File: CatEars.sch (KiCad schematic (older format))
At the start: 14 parts, among them J0 Conn_01x03_Female, J1 Conn_01x03_Female

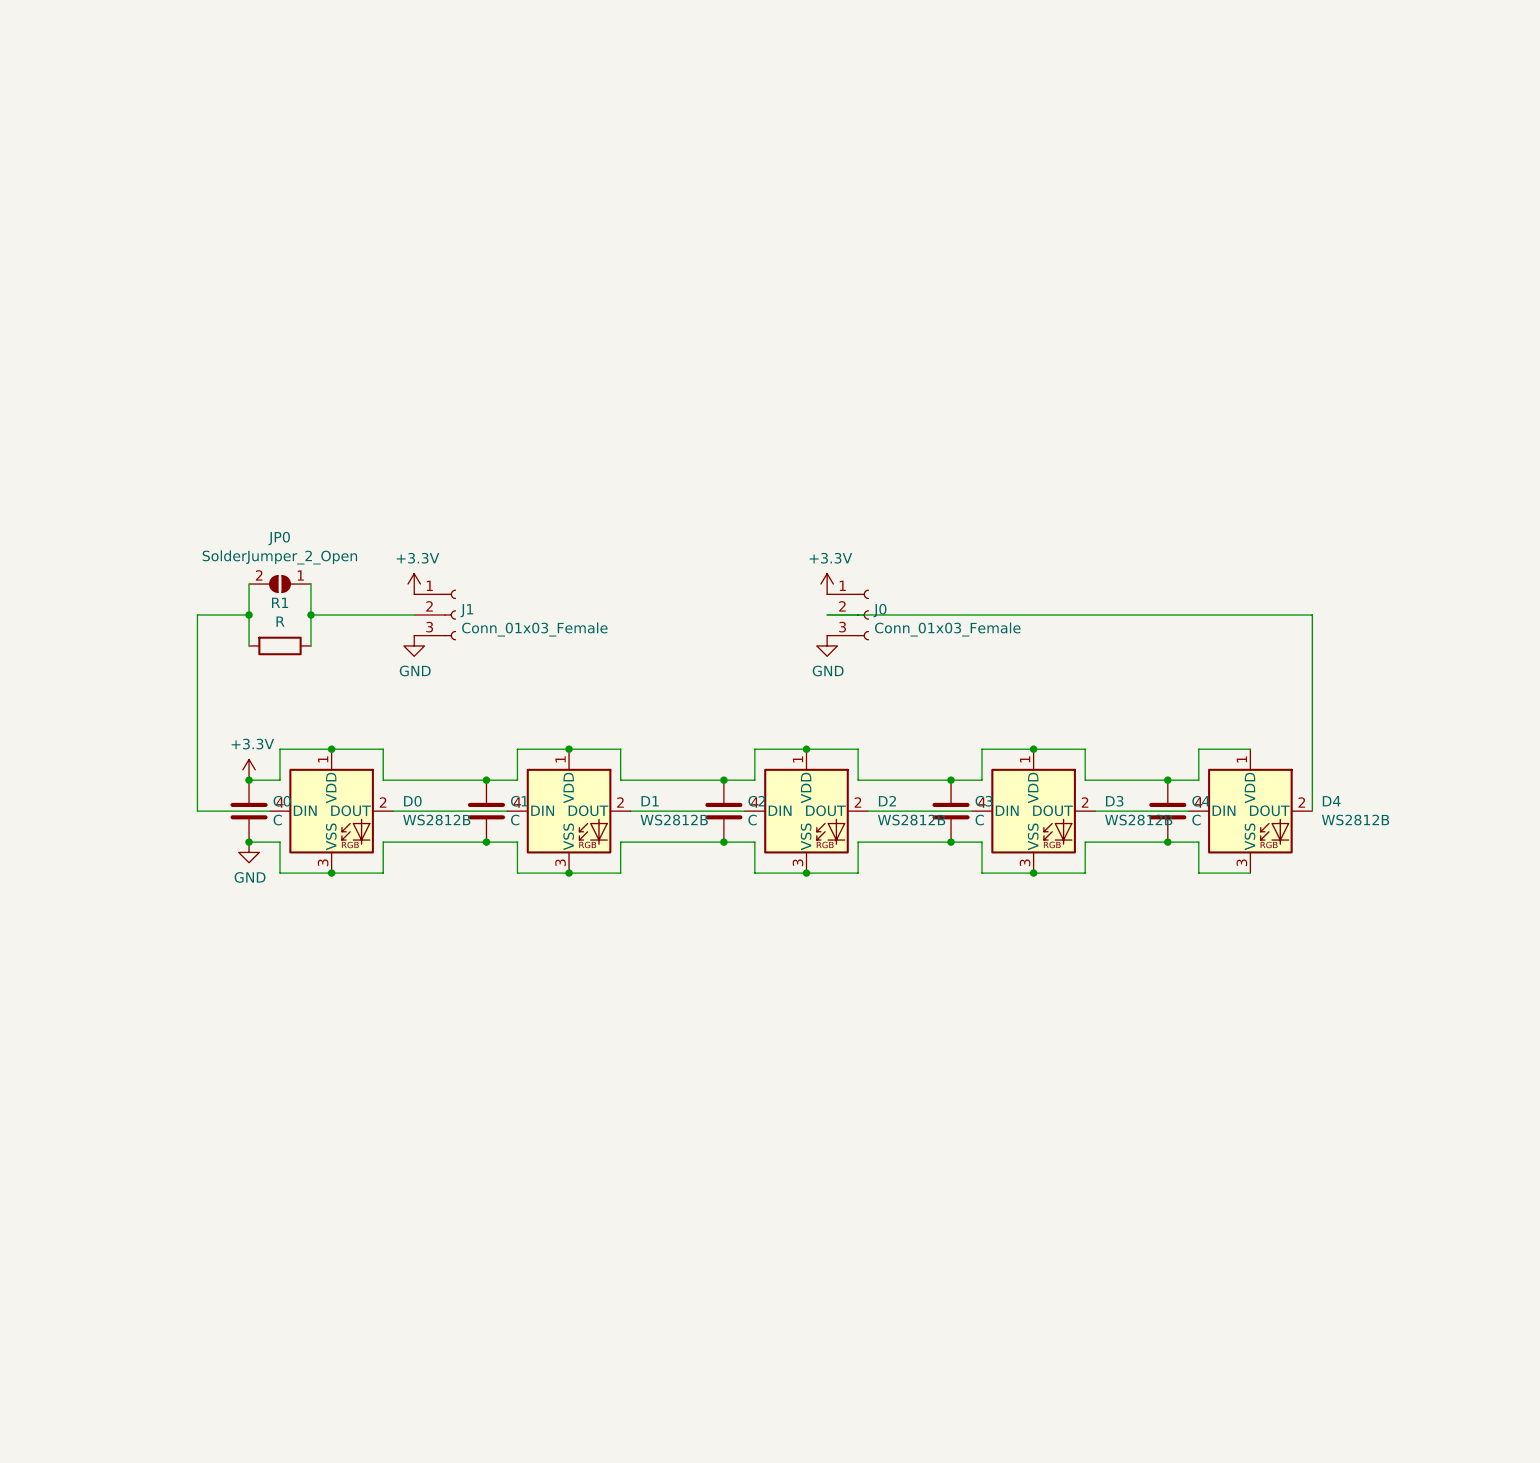
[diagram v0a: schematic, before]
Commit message: Added schematic and copper
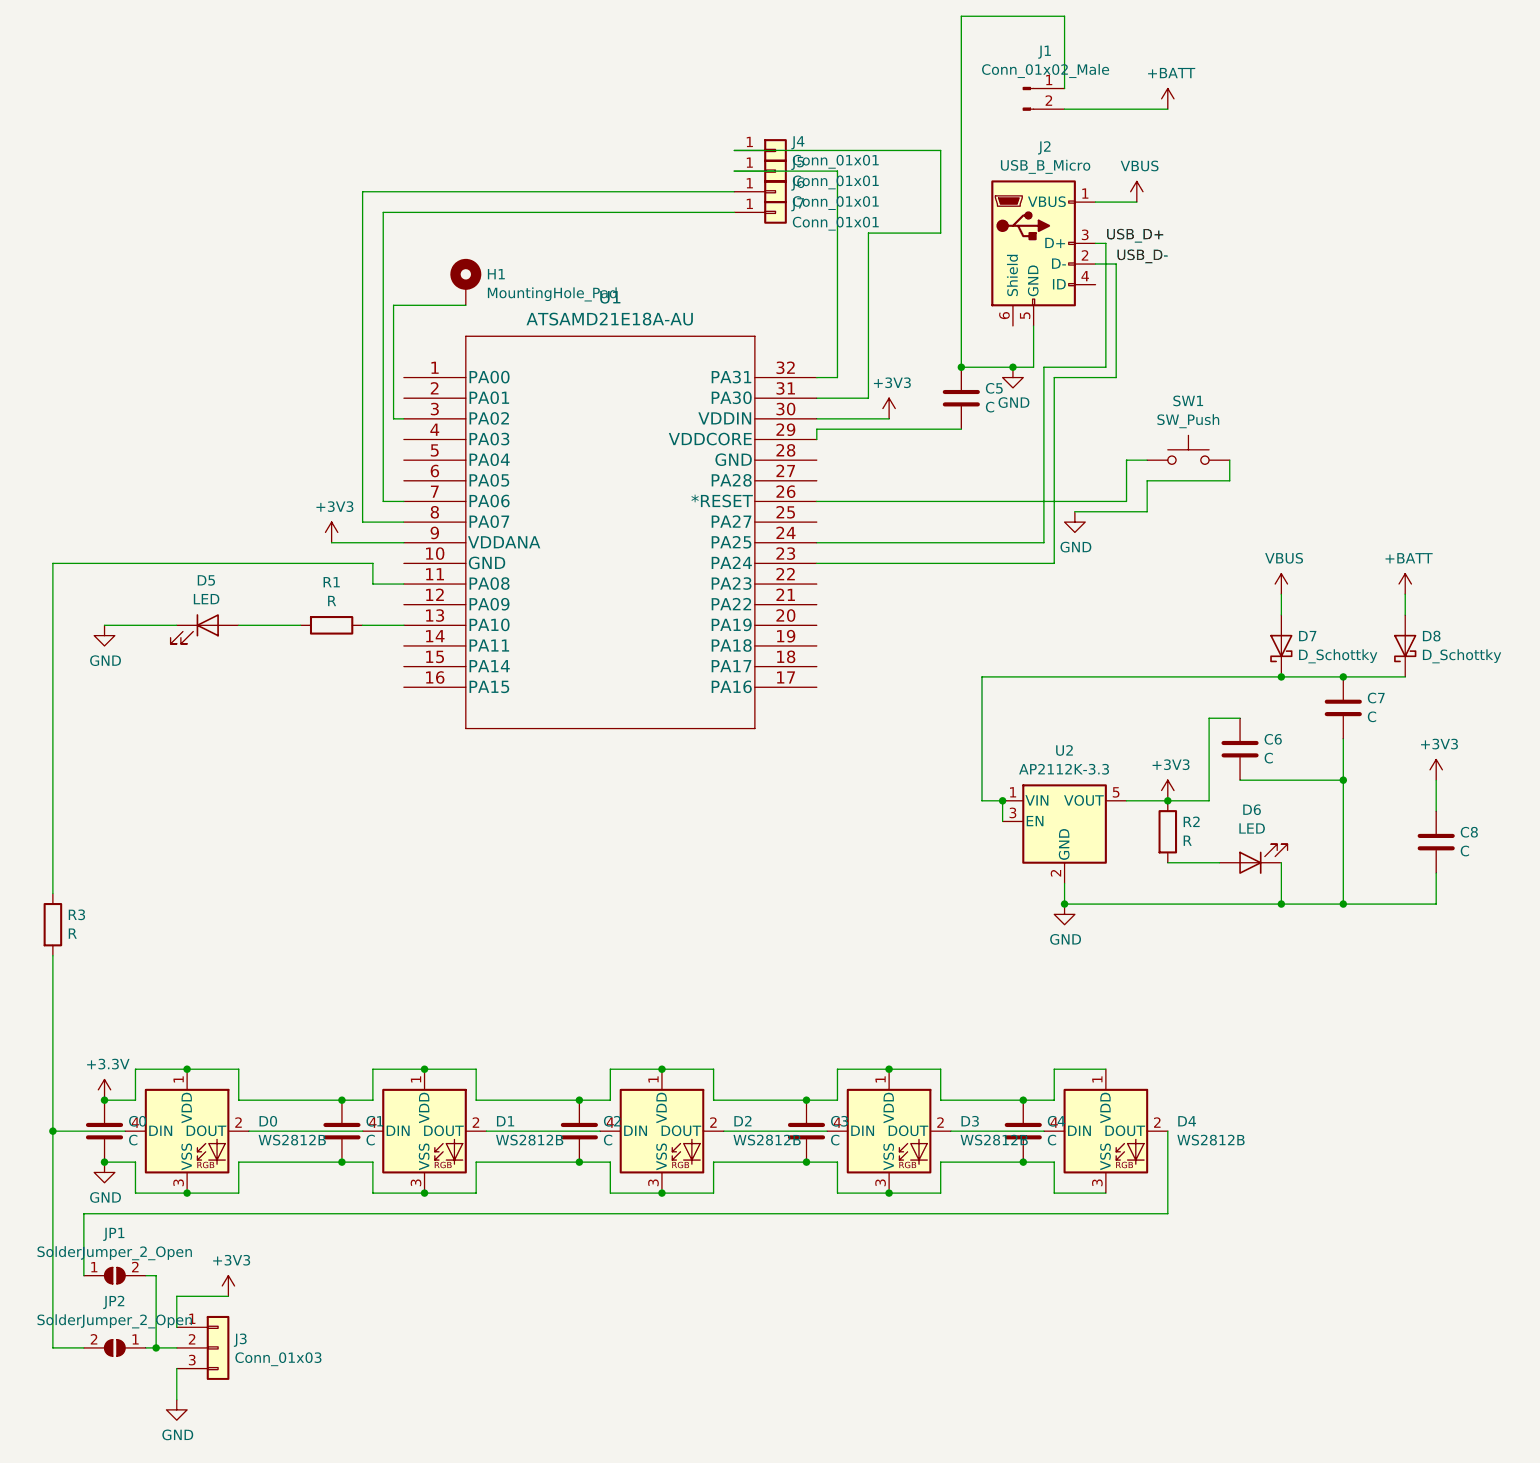
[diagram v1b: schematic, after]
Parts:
- removed J0, J1: Conn_01x03_Female, Connector_PinSocket_2.54mm:PinSocket_1x03_P2.54mm_Vertical, symbol Connector:Conn_01x03_Female
- removed JP0: SolderJumper_2_Open, Jumper:SolderJumper-2_P1.3mm_Open_TrianglePad1.0x1.5mm, symbol Jumper:SolderJumper_2_Open
- added C5, C6, C7, C8: C, Capacitor_SMD:C_0603_1608Metric_Pad1.05x0.95mm_HandSolder, symbol Device:C
- added D5, D6: LED, LED_SMD:LED_0805_2012Metric_Pad1.15x1.40mm_HandSolder, symbol Device:LED
- added D7, D8: D_Schottky, Diode_SMD:D_SOT-23_ANK, symbol Device:D_Schottky
- added H1: MountingHole_Pad, TestPoint:TestPoint_Pad_D1.5mm, symbol Mechanical:MountingHole_Pad
- added J1: Conn_01x02_Male, Connector_JST:JST_PH_B2B-PH-K_1x02_P2.00mm_Vertical, symbol Connector:Conn_01x02_Male
- added J2: USB_B_Micro, Connector_USB:USB_Micro-B_GCT_USB3076-30-A, symbol Connector:USB_B_Micro
- added J3: Conn_01x03, Connector_PinSocket_2.54mm:PinSocket_1x03_P2.54mm_Vertical, symbol Connector_Generic:Conn_01x03
- added J4, J5, J6, J7: Conn_01x01, TestPoint:TestPoint_Pad_D1.0mm, symbol Connector_Generic:Conn_01x01
- added JP1, JP2: SolderJumper_2_Open, Jumper:SolderJumper-2_P1.3mm_Open_TrianglePad1.0x1.5mm, symbol Jumper:SolderJumper_2_Open
- added R2, R3: R, Resistor_SMD:R_0805_2012Metric_Pad1.15x1.40mm_HandSolder, symbol Device:R
- added SW1: SW_Push, Button_Switch_SMD:SW_SPST_TL3342, symbol Switch:SW_Push
- added U1: ATSAMD21E18A-AU, Package_QFP:TQFP-32_7x7mm_P0.8mm, symbol 2020-01-10_20-18-23:ATSAMD21E18A-AU
- added U2: AP2112K-3.3, Package_TO_SOT_SMD:SOT-23-5, symbol Regulator_Linear:AP2112K-3.3
- R1: footprint Capacitor_SMD:C_0805_2012Metric_Pad1.15x1.40mm_HandSolder -> Resistor_SMD:R_0805_2012Metric_Pad1.15x1.40mm_HandSolder
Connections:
- net +3V3: now also C6.1, C8.1, J3.1 (Pin_1), R2.1, U1.30 (VDDIN), U1.9 (VDDANA), U2.5 (VOUT)
- net GND: now also C5.1, C6.2, C7.2, C8.2, D5.1 (K), D6.1 (K), J1.1 (Pin_1), J2.5 (GND), J3.3 (Pin_3), SW1.2, U2.2 (GND)
- net at R1.1: now also U1.13 (PA10)
- net at D4.2 (DOUT): now also JP1.1 (A)
- net at D0.4 (DIN): now also JP2.2 (B), R3.2; no longer R1.2
- new net: C7.1, D7.1 (K), D8.1 (K), U2.1 (VIN), U2.3 (EN)
- new net: R3.1, U1.11 (PA08)
- new net: SW1.1, U1.26 (*RESET)
- new net: C5.2, U1.29 (VDDCORE)
- new net: H1.1, U1.3 (PA02)
- new net: J4.1 (Pin_1), U1.31 (PA30)
- new net: J5.1 (Pin_1), U1.32 (PA31)
- new net: J7.1 (Pin_1), U1.7 (PA06)
- new net: J6.1 (Pin_1), U1.8 (PA07)
- new net: D5.2 (A), R1.2
- new net: D6.2 (A), R2.2
- new net: J3.2 (Pin_2), JP1.2 (B), JP2.1 (A)
- new net +BATT: D8.2 (A), J1.2 (Pin_2)
- new net USB_D+: J2.3 (D+), U1.24 (PA25)
- new net USB_D-: J2.2 (D-), U1.23 (PA24)
- new net VBUS: D7.2 (A), J2.1 (VBUS)
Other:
- moved on the sheet: C0, C1, C2, C3, C4, D0, D1, D2, D3, D4
